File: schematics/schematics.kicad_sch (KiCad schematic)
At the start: 22 parts

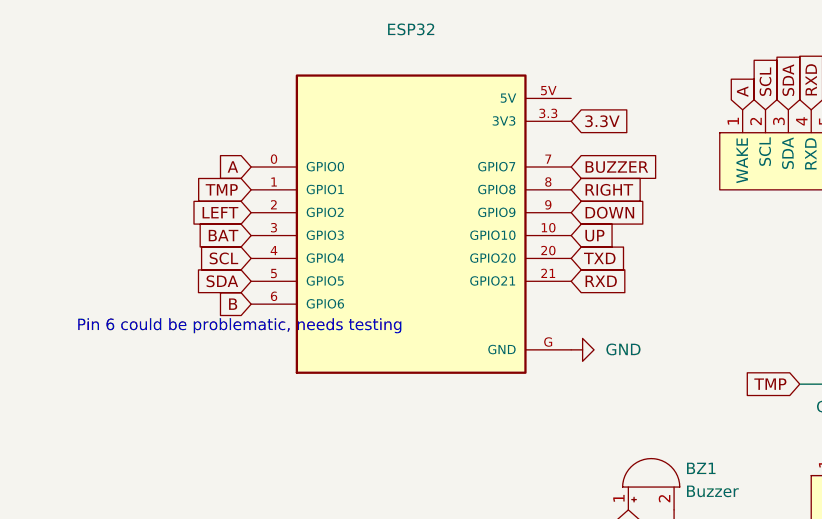
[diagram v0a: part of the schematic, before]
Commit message: Real code for the real version of the board
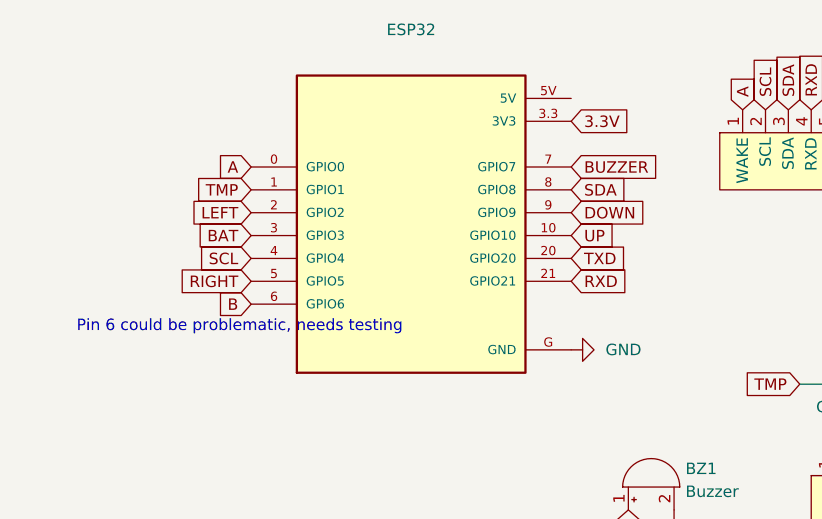
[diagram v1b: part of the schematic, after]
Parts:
- BAT1: footprint custom:LIPOBattery Header -> custom:PowerHeader BACKSIDE
- BZ1: footprint Buzzer_Beeper:Buzzer_12x9.5RM7.6 -> Buzzer_Beeper:MagneticBuzzer_StarMicronics_QMX
- POW1: footprint custom:LIPOBattery Header -> custom:PowerHeader
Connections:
- net RIGHT: now also ESP32.5 (GPIO5); no longer ESP32.8 (GPIO8)
- net SDA: now also ESP32.8 (GPIO8); no longer ESP32.5 (GPIO5)
